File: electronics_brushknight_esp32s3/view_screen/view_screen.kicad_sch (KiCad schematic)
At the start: 12 parts, among them J1 Conn_01x04, J2 GC9A01, J3 Conn_01x04, J4 Conn_01x04, J5 Conn_01x04, Q1 2N7002

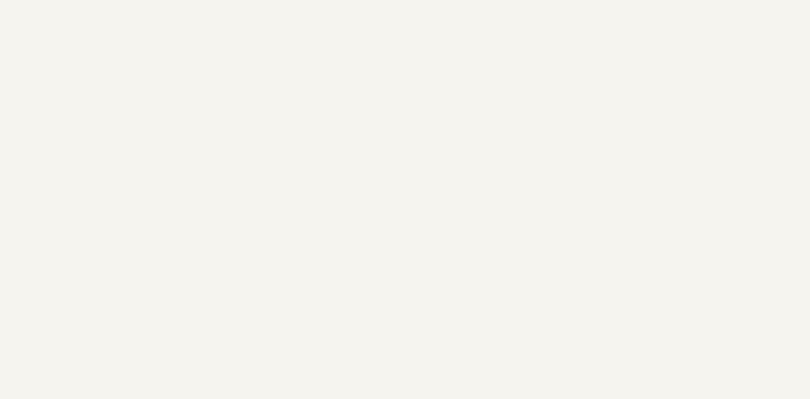
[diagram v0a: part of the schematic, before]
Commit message: devkit pcb preview
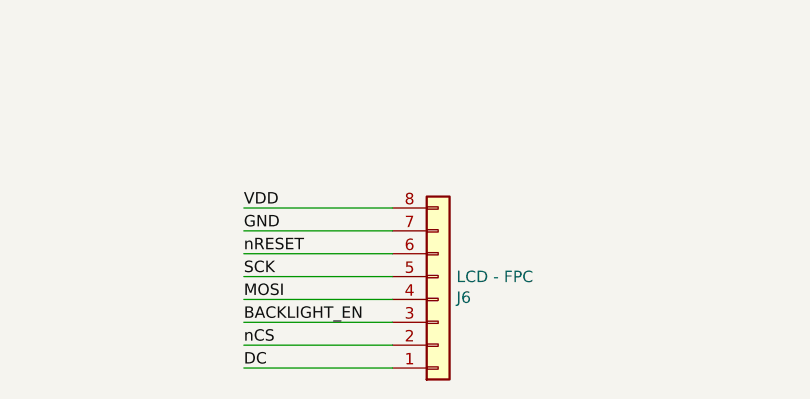
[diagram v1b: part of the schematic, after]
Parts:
- added J6: LCD - FPC, screen_connector:Amphenol FCI FPC 8 pin 0.5 pitch, symbol Connector_Generic:Conn_01x08
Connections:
- net BACKLIGHT_EN: now also J6.3 (Pin_3)
- net DC: now also J6.1 (Pin_1)
- net GND: now also J6.7 (Pin_7)
- net MOSI: now also J6.4 (Pin_4)
- net SCK: now also J6.5 (Pin_5)
- net VDD: now also J6.8 (Pin_8)
- net nCS: now also J6.2 (Pin_2)
- net nRESET: now also J6.6 (Pin_6)
